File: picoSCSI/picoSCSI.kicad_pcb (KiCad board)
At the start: 2 copper layers, 100 x 90 mm, 19 parts, among them J1 SCSI_CONN, J2 Micro_SD_Card, J3 Floppy Power

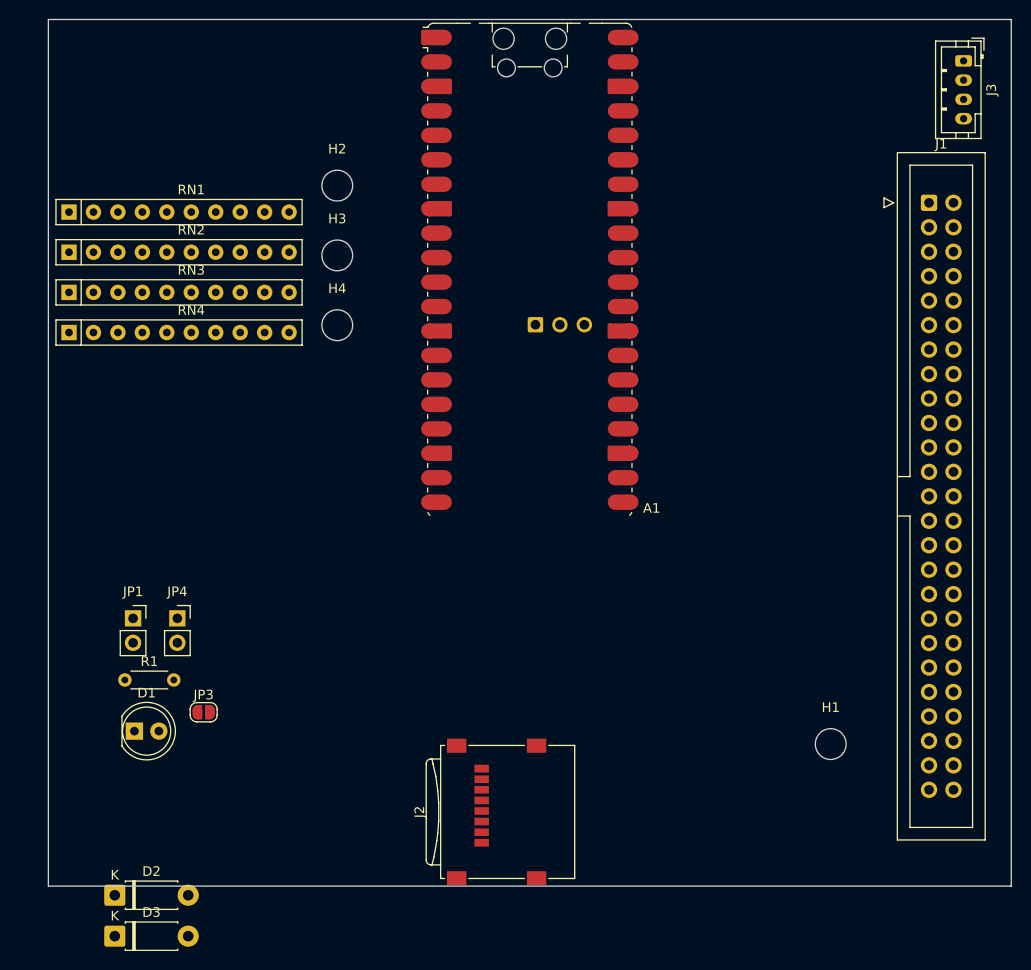
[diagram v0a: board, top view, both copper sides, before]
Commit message: tmp
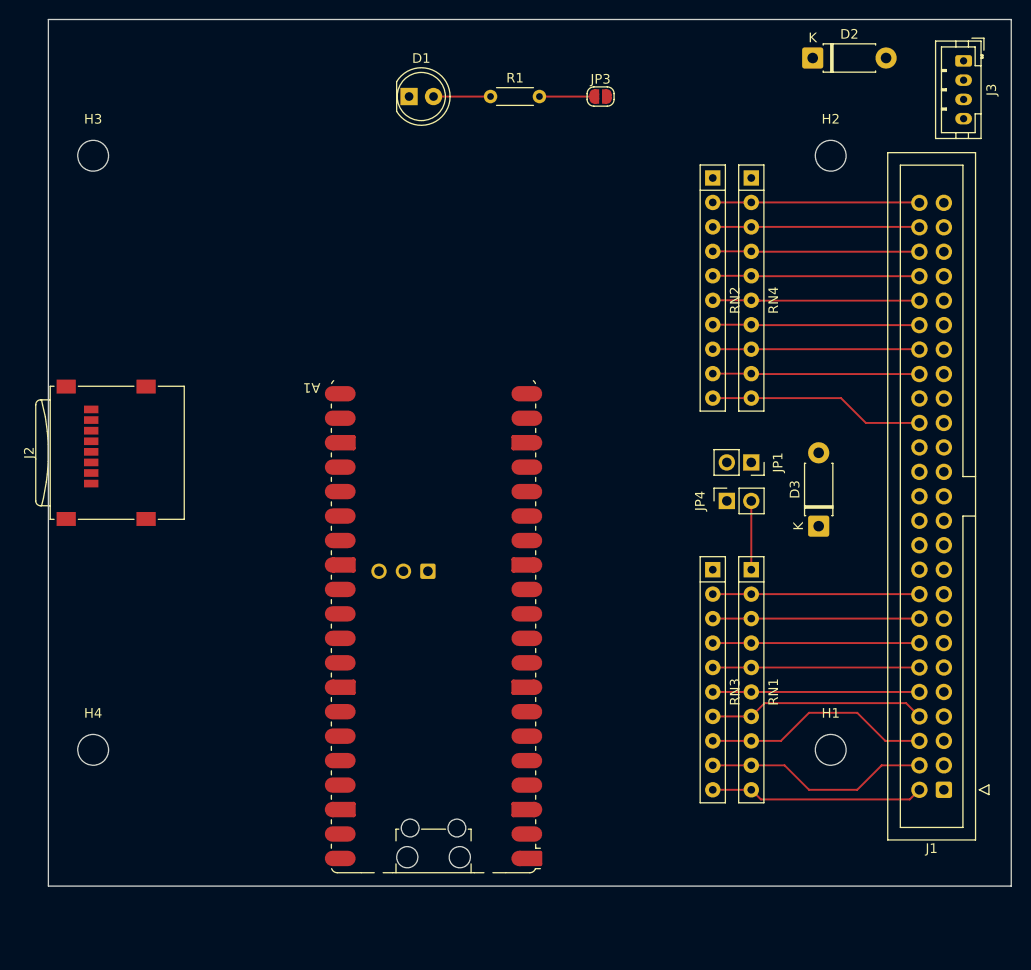
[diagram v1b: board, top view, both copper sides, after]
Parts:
- moved D2 113.2 mm to (108.1, 42.5)
- moved D3 84.6 mm to (108.8, 91.1), turned to 90 degrees
- moved RN1 80.0 mm to (101.8, 95.6), turned to -90 degrees
- moved JP3 76.1 mm to (86.1, 46.5)
- moved RN3 72.8 mm to (97.8, 95.6), turned to -90 degrees
- moved RN4 72.7 mm to (101.8, 55.0), turned to -90 degrees
- moved D1 71.8 mm to (66.2, 46.5)
- moved R1 71.5 mm to (74.7, 46.5)
- moved RN2 67.3 mm to (97.8, 55.0), turned to -90 degrees
- moved JP1 66.2 mm to (101.8, 84.5), turned to -90 degrees
- moved J1 61.0 mm to (121.8, 118.5), turned to 180 degrees
- moved JP4 58.4 mm to (99.2, 88.5), turned to 90 degrees
- moved J2 55.1 mm to (34.8, 83.5)
- moved H2 51.3 mm to (110.0, 52.6)
- moved H4 50.9 mm to (33.4, 114.3)
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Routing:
- net /SCSI_DATA2: track 0.00 -> 23.9 mm
- net /SCSI_DATA1: track 0.00 -> 23.6 mm
- net /SCSI_DATA3: track 0.00 -> 22.6 mm
- net /SCSI_ATN: track 0.00 -> 22.5 mm
- net /SCSI_DATA0: track 0.00 -> 22.3 mm
- net /SCSI_MSG: track 0.00 -> 21.5 mm
- net /SCSI_ACK: track 0.00 -> 21.5 mm
- net /SCSI_REQ: track 0.00 -> 21.5 mm
- net /SCSI_IO: track 0.00 -> 21.5 mm
- net /SCSI_CD: track 0.00 -> 21.5 mm
- net /SCSI_SEL: track 0.00 -> 21.5 mm
- net /SCSI_RST: track 0.00 -> 21.5 mm
- net /SCSI_BSY: track 0.00 -> 21.5 mm
- net /SCSI_DATA7: track 0.00 -> 21.5 mm
- net /SCSI_DATA6: track 0.00 -> 21.5 mm
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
